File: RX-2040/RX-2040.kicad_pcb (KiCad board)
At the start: 4 copper layers, 9.3 x 2.2 mm, 20 parts, among them J1 UJ31-CH-31-SMT-TR, U1 NCP1117-3.3_SOT223, U2 RP2040

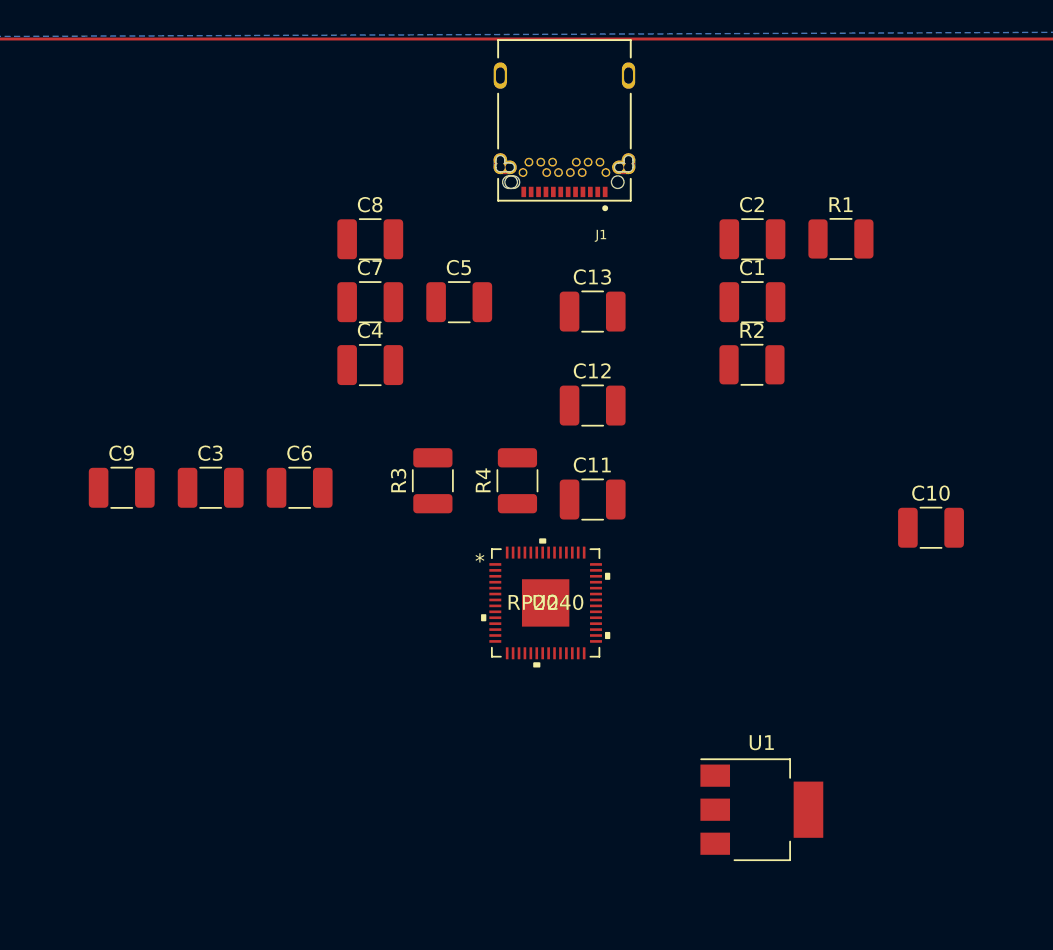
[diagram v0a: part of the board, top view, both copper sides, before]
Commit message: Deleting previous work, starting over
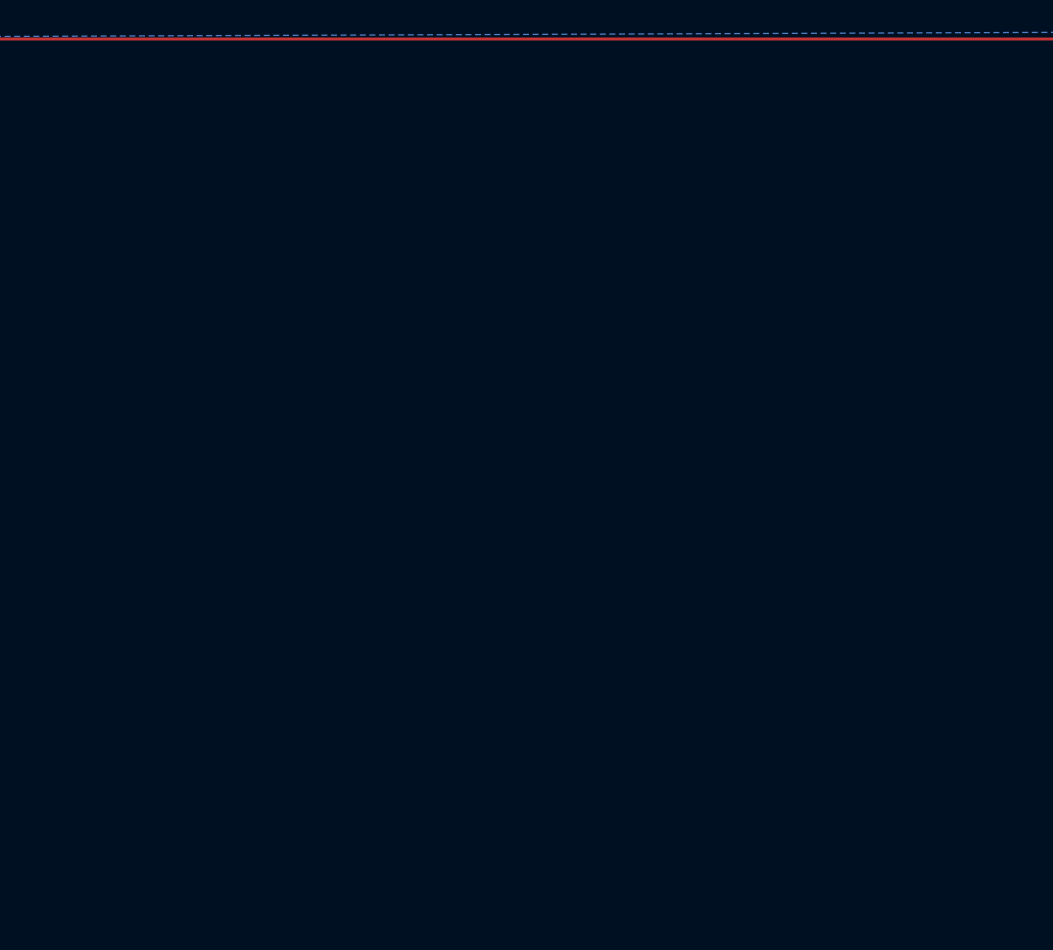
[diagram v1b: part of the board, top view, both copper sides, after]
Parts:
- removed C1, C2, C4: 10μf, Capacitor_SMD:C_1210_3225Metric_Pad1.33x2.70mm_HandSolder
- removed C10, C12, C13, C3, C5, C6, C7, C8, C9: 100nf, Capacitor_SMD:C_1210_3225Metric_Pad1.33x2.70mm_HandSolder
- removed C11: 1μf, Capacitor_SMD:C_1210_3225Metric_Pad1.33x2.70mm_HandSolder
- removed J1: UJ31-CH-31-SMT-TR, UJ31-CH-31-SMT-TR:CUI_UJ31-CH-31-SMT-TR
- removed R1, R2: 5.1k, Resistor_SMD:R_1210_3225Metric_Pad1.30x2.65mm_HandSolder
- removed R3, R4: 27.4, Resistor_SMD:R_1210_3225Metric_Pad1.30x2.65mm_HandSolder
- removed U1: NCP1117-3.3_SOT223, Package_TO_SOT_SMD:SOT-223-3_TabPin2
- removed U2: RP2040, RP2040:RP2040
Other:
- board outline removed
